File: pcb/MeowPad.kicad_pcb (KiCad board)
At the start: 2 copper layers, 71 x 97.5 mm, 57 parts, among them M1 MOUDLE-SEEEDUINO-XIAO

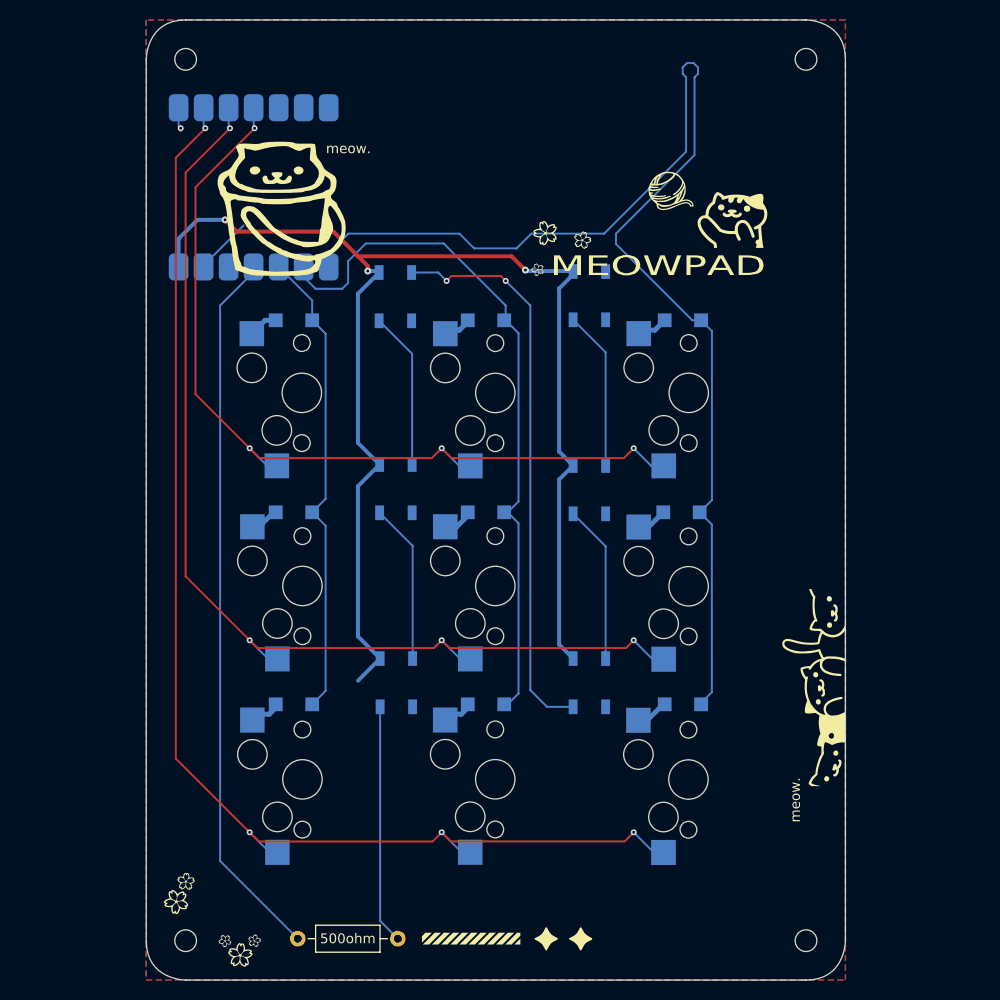
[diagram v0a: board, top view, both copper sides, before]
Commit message: Update PCB
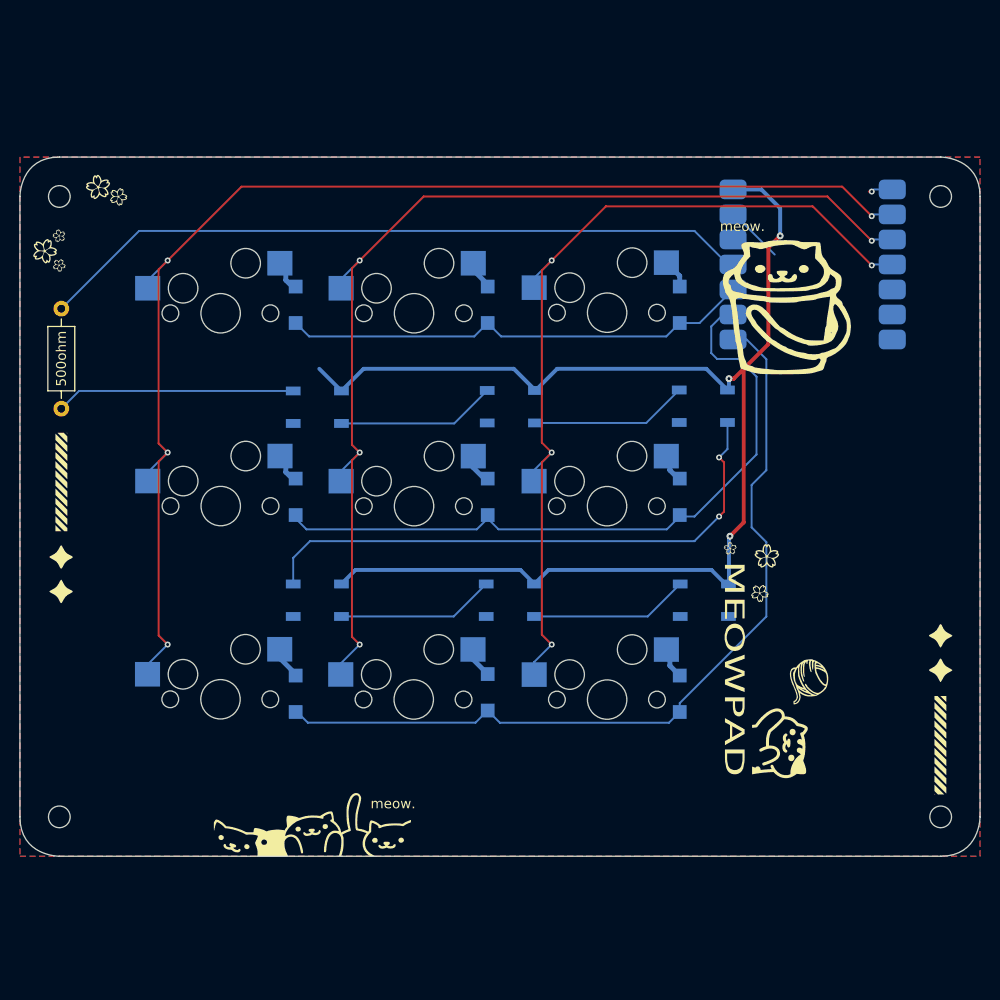
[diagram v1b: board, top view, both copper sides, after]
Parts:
- added G***: LOGO, LOGO, F.Cu at (177.4, 106.5)
- added G***: LOGO, LOGO, F.Cu at (177.4, 117.5)
- added G***: LOGO, LOGO, F.Cu at (177.4, 110.0)
- moved REF** 78.1 mm to (177.4, 124.8), turned to 0 degrees
- moved REF** 77.9 mm to (177.4, 61.8), turned to 0 degrees
- moved REF** 76.9 mm to (87.9, 124.8), turned to 0 degrees
- moved REF** 76.7 mm to (87.9, 61.8), turned to 0 degrees
- moved G*** 76.4 mm to (86.1, 64.8), turned to 40 degrees
- moved G*** 74.3 mm to (86.4, 67.3), turned to 50 degrees
- moved G*** 74.0 mm to (91.6, 60.0), turned to -25 degrees
- moved G*** 73.8 mm to (87.1, 66.8), turned to 80 degrees
- moved G*** 73.6 mm to (87.9, 65.8), turned to 85 degrees
- moved G*** 73.0 mm to (91.9, 60.8), turned to 10 degrees
- moved G*** 71.9 mm to (93.1, 60.5), turned to -65 degrees
- moved G*** 71.7 mm to (92.1, 62.0), turned to 40 degrees
- moved G*** 71.4 mm to (87.9, 68.8), turned to 115 degrees
- moved G*** 70.0 mm to (93.9, 61.8), turned to 50 degrees
- moved R1 68.3 mm to (88.1, 73.2), turned to -90 degrees
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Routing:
- net ROW2: track 128.0 -> 85.9 mm
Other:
- board size 71 x 97.5 mm -> 97.5 x 71 mm
- board text added: "meow meow meow meow meow meow meow meow meow meow meow meow meow meow meow meow meow meow meow meow meow meow meow meow meow meow meow meow meow meow meow meow meow meow meow meow meow meow meow meow meow meow meow meow meow meow meow meow meow meow meow meow meow meow meow"
- board text removed: "meow meow meow meow meow meow meow meow meow meow meow meow meow meow meow meow meow meow meow meow meow meow meow meow meow meow meow meow meow meow meow meow meow meow meow meow meow meow meow meow meow meow meow meow meow meow meow meow meow meow meow meow meow meow meow meow meow meow meow meow meow meow meow meow meow meow meow meow meow meow meow meow meow meow meow meow meow meow meow meow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"
